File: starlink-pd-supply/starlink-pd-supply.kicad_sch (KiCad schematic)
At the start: 62 parts

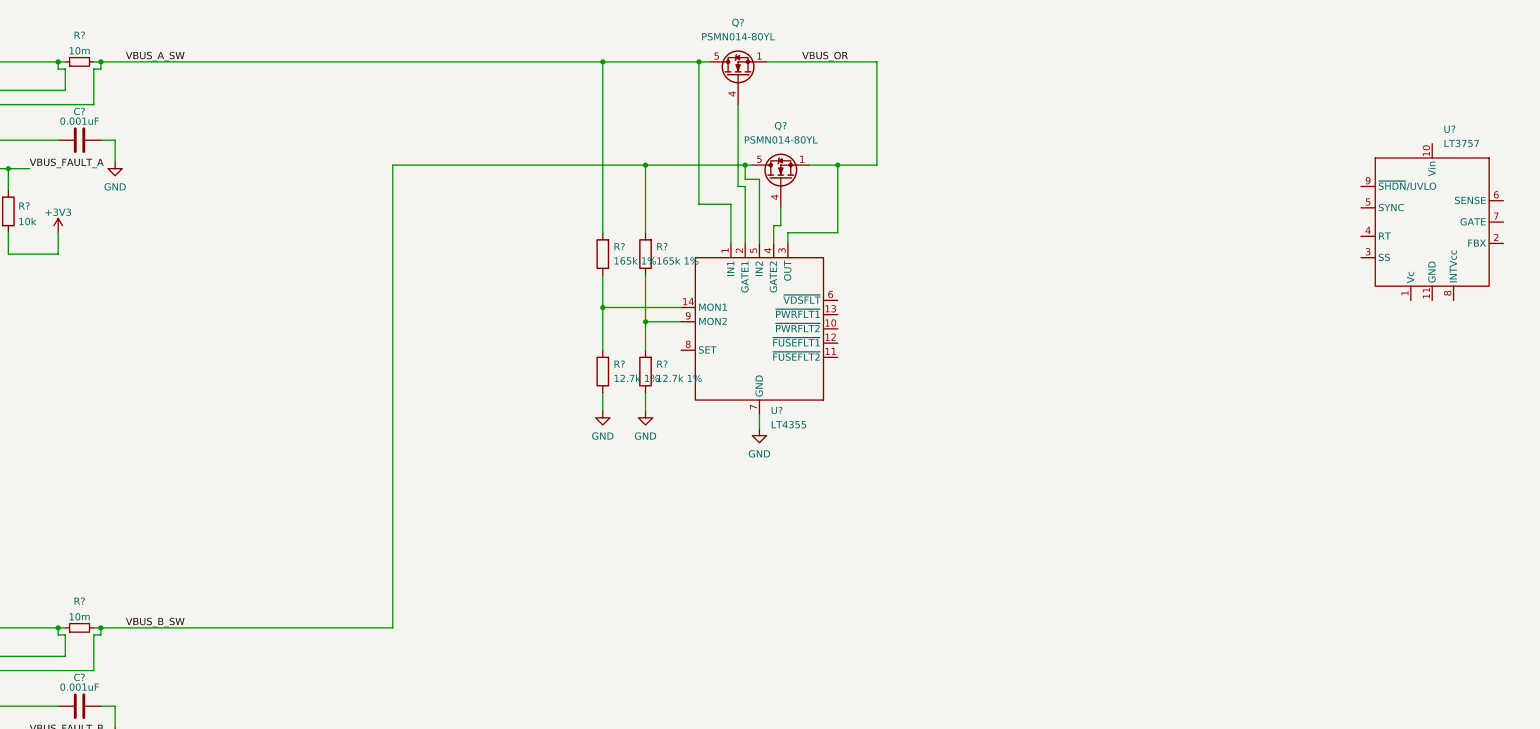
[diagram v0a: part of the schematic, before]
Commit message: WIP
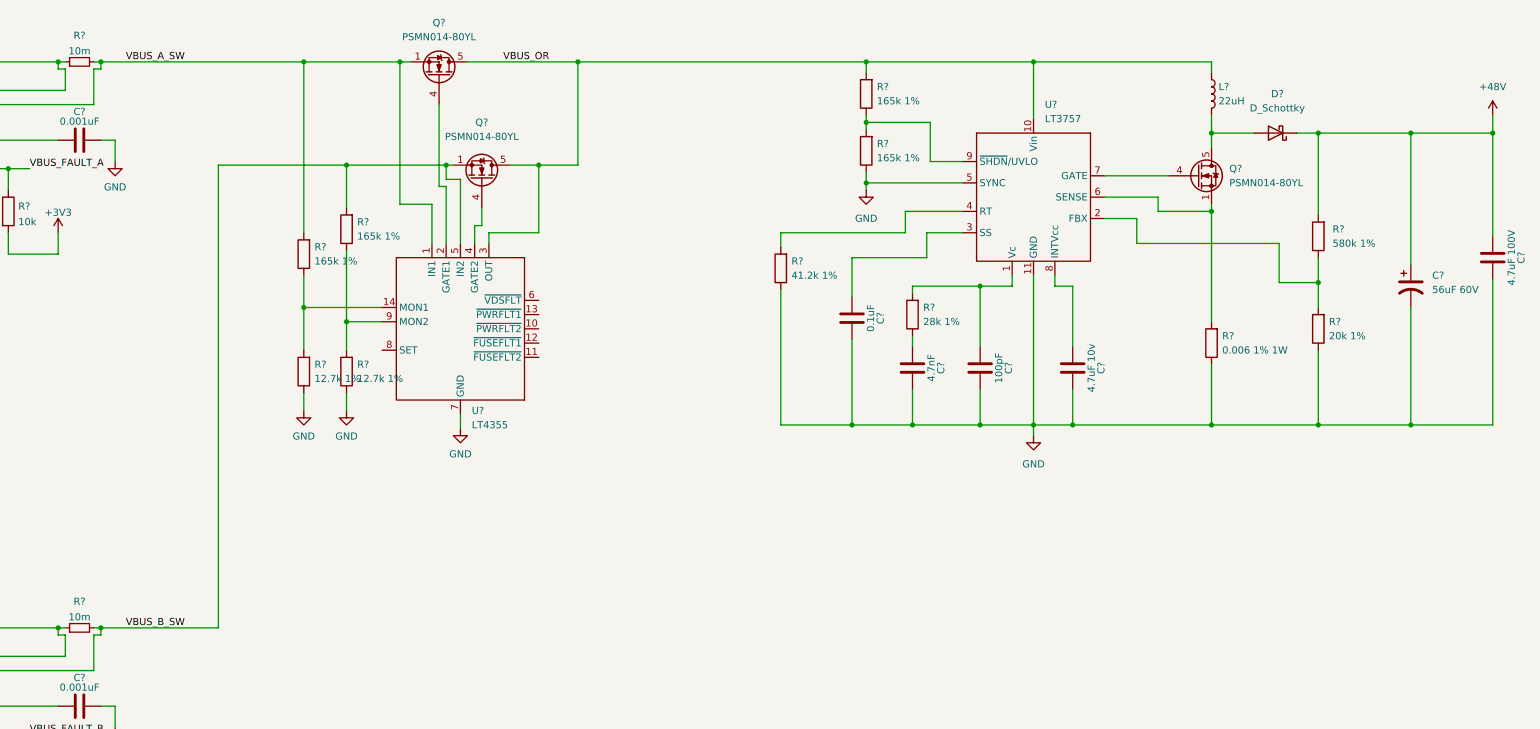
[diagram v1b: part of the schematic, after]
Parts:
- added C?: 4.7uF 10v, Capacitor_SMD:C_0805_2012Metric, symbol Device:C
- added C?: 0.1uF, Capacitor_SMD:C_0805_2012Metric, symbol Device:C
- added C?: 56uF 60V, symbol Device:C_Polarized_US
- added C?: 4.7uF 100V, Capacitor_SMD:C_0805_2012Metric, symbol Device:C
- added C?: 100pF, Capacitor_SMD:C_0805_2012Metric, symbol Device:C
- added C?: 4.7nF, Capacitor_SMD:C_0805_2012Metric, symbol Device:C
- added D?: D_Schottky, symbol Device:D_Schottky
- added L?: 22uH, symbol Device:L
- added Q?: PSMN014-80YL, Package_TO_SOT_SMD:LFPAK56, symbol Custom:PSMN014-80YL
- added R? (x2): 165k 1%, Resistor_SMD:R_0805_2012Metric, symbol Device:R
- added R?: 0.006 1% 1W, Resistor_SMD:R_0805_2012Metric, symbol Device:R
- added R?: 28k 1%, Resistor_SMD:R_0805_2012Metric, symbol Device:R
- added R?: 20k 1%, Resistor_SMD:R_0805_2012Metric, symbol Device:R
- added R?: 580k 1%, Resistor_SMD:R_0805_2012Metric, symbol Device:R
- added R?: 41.2k 1%, Resistor_SMD:R_0805_2012Metric, symbol Device:R
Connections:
- net GND: now also U?.11 (GND), U?.5 (SYNC), C?.2, C?.2, C?.2, C?.2, C?.2, C?.2, R?.1, R?.1, R?.1, R?.1
- net VBUS_A_SW: now also Q?.1 (S), Q?.2 (S), Q?.3 (S); no longer Q?.5 (D)
- net VBUS_B_SW: now also Q?.1 (S), Q?.2 (S), Q?.3 (S); no longer Q?.5 (D)
- net VBUS_OR: now also Q?.5 (D), Q?.5 (D), U?.10 (Vin), L?.1, R?.2; no longer Q?.1 (S), Q?.1 (S), Q?.2 (S), Q?.2 (S), Q?.3 (S), Q?.3 (S)
- net at U?.1 (Vc): now also C?.1, R?.2
- net at U?.2 (FBX): now also R?.1, R?.2
- net at U?.3 (SS): now also C?.1
- net at U?.4 (RT): now also R?.2
- net at U?.6 (SENSE): now also Q?.1 (S), Q?.2 (S), Q?.3 (S), R?.2
- net at U?.7 (GATE): now also Q?.4 (G)
- net at U?.8 (INTVcc): now also C?.1
- net at U?.9 (~{SHDN}/UVLO): now also R?.1, R?.2
- new net: D?.2 (A), L?.2, Q?.5 (D)
- new net: C?.1, R?.1
- new net +48V: C?.1, C?.1, D?.1 (K), R?.2
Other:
- moved on the sheet: Q?, R?, U?
